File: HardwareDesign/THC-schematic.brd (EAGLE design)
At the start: 45 x 83 mm, 41 parts

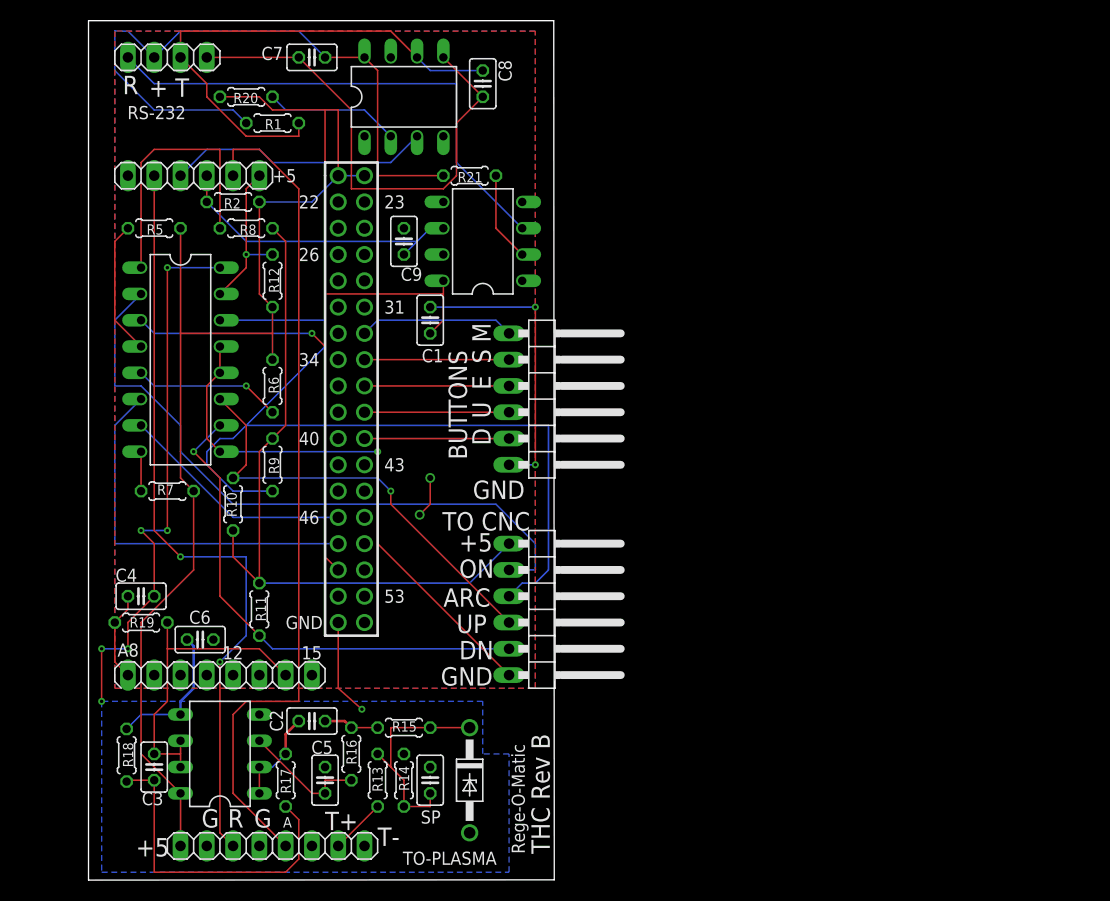
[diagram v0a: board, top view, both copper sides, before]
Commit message: Rev C Hardware
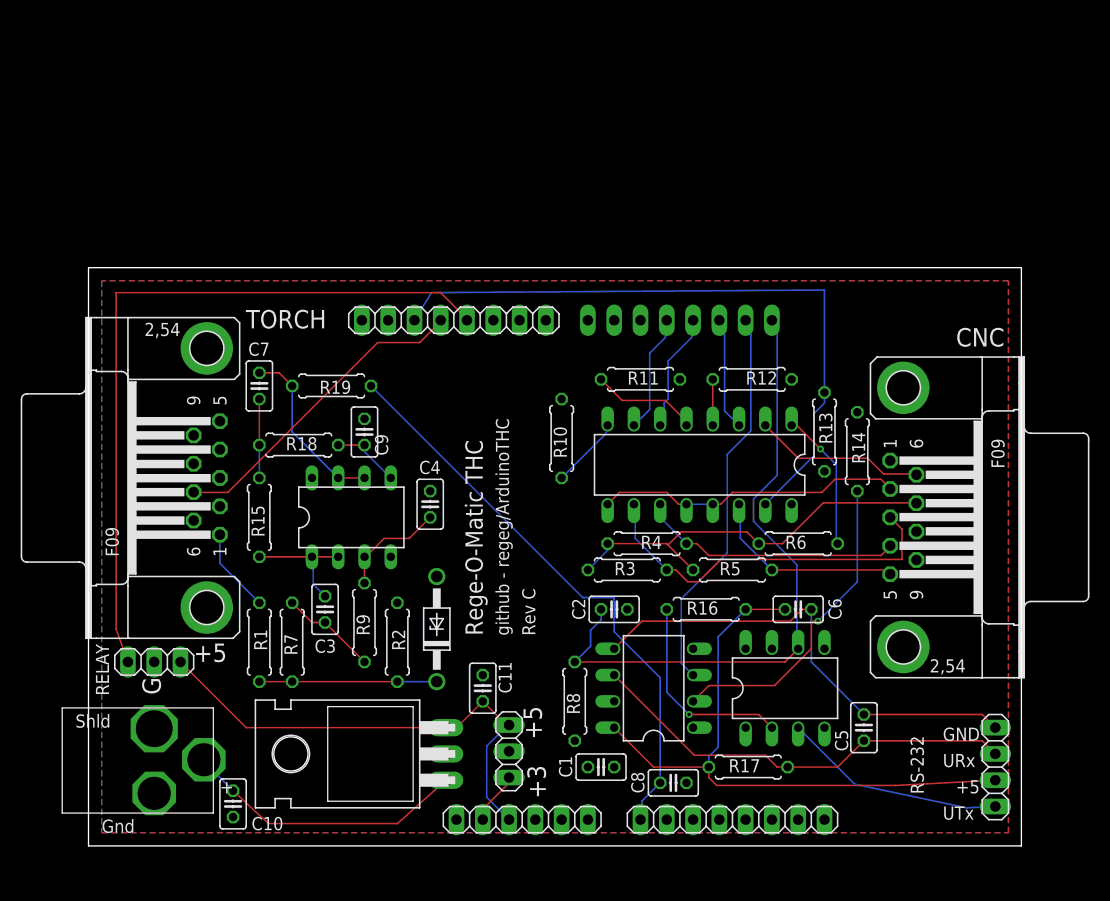
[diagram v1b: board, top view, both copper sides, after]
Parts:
- removed ARDUNIO-COMM: JJ, pinhead:1X06
- removed BUTTONS: CON1, pinhead:1X06/90
- removed MEGA-IO: ARDUINO-MEGA-18X2, ArduinoConnect18x2:CONN-18X2
- removed OK4: 6N137, optocoupler:DIL08
- removed R20, R21: 560, resistor:0204/5
- removed SP: 0, resistor:C025-025X050
- removed TO-CNC: CON3, pinhead:1X06/90
- removed TO-PLASMA: J1, pinhead:1X08
- removed U$2: LT1632, ArduinoThcOpAmp:DIP08
- added ARD-ANALOG, ARD-PWM, JP1: (no value), pinhead:1X08
- added ARD-PWR: (no value), pinhead:1X06
- added C10: 100nF / .1 uF, resistor:C025-025X050
- added C11: 100 nF / .1 uF, resistor:C025-025X050
- added CNC, TORCH: (no value), con-subd:F09HP
- added IC1: 7805T, adafruit:TO220H
- added ILQ2: ILQ1, optocoupler:DIL16
- added J1: 2.1MM-PLUG-PCB-MNT, ArdunioPowerJack:2.1MM-PLUG
- added JP2, RELAY: (no value), pinhead:1X03
- added R3, R4: 1k, resistor:0207/7
- C1: value .1uF -> 100 nF / 0.1uF
- C2: value 150n -> 15pf
- C3: value 1u -> 150 nf
- C4: value 10uF -> 100 nf / 0.1 uF
- C5: value 100n -> 15pf
- C6: value 100n -> 100 nF / 0.1uF
- C7: value .1uF -> 1 uF
- C8: value 15pf -> 10 uF
- C9: value 15pf -> 100 nf
- OK2: value ILQ1 -> 6N137; device optocoupler:DIL16 -> optocoupler:DIL08
- R1: value 350 -> 220k; device resistor:0204/5 -> resistor:0207/7
- R10, R11, R12: value 1k -> 560; device resistor:0204/5 -> resistor:0207/7
- R13: value 220k -> 1k; device resistor:0204/5 -> resistor:0207/7
- R14: value 15k -> 560; device resistor:0204/5 -> resistor:0207/7
- R15: value 7.87k -> 2.61k; device resistor:0204/5 -> resistor:0207/7
- R16: value 21.5k -> 560; device resistor:0204/5 -> resistor:0207/7
- R17: value 2.61k -> 350; device resistor:0204/5 -> resistor:0207/7
- R18, R19, R6: device resistor:0204/5 -> resistor:0207/7
- R2: value 350 -> 15k; device resistor:0204/5 -> resistor:0207/7
- R5: value 560 -> 1k; device resistor:0204/5 -> resistor:0207/7
- R7: value 560 -> 7.87k; device resistor:0204/5 -> resistor:0207/7
- R8: value 560 -> 350; device resistor:0204/5 -> resistor:0207/7
- R9: value 1k -> 21.5k; device resistor:0204/5 -> resistor:0207/7
- U$1: value PIN-ARD-A8 -> LT1632; device Rege:A8-1X8 -> ArduinoThcOpAmp:DIP08
- moved RS-232 105.4 mm to (87.6, 7.62), turned to 90 degrees
- moved C8 70.0 mm to (56.5, 6.10), turned to 0 degrees
- moved OK2 66.5 mm to (67.3, 15.2), turned to 0 degrees
- moved R5 64.9 mm to (62.2, 26.7)
- moved OK3 62.0 mm to (54.6, 15.2), turned to 90 degrees
- moved C6 57.9 mm to (68.6, 22.9)
- moved R8 55.7 mm to (47.0, 14.0), turned to 90 degrees
- moved R13 54.7 mm to (71.1, 40.0), turned to 270 degrees
- moved R14 54.1 mm to (74.3, 38.1)
- moved R6 53.0 mm to (68.6, 29.2), turned to 0 degrees
- moved C5 52.3 mm to (74.9, 11.4)
- moved R1 50.2 mm to (16.5, 19.7), turned to 270 degrees
- moved R12 47.3 mm to (64.1, 45.1), turned to 0 degrees
- moved C1 46.2 mm to (49.5, 7.62), turned to 0 degrees
- moved R2 45.4 mm to (29.8, 19.7), turned to 270 degrees
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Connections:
- removed net N$14: BUTTONS.1, MEGA-IO.D-33
- removed net N$15: BUTTONS.2, MEGA-IO.D-35
- removed net N$17: MEGA-IO.D-50, OK2.3
- removed net N$18: MEGA-IO.D-48, OK2.6
- removed net N$19: MEGA-IO.D-46, OK2.7
- removed net N$23: BUTTONS.3, MEGA-IO.D-37
- removed net N$24: BUTTONS.4, MEGA-IO.D-39
- removed net N$25: BUTTONS.5, MEGA-IO.D-41
- removed net N$28: C4.1, R19.1, U$1.1
- new net +3.3V: ARD-PWR.5, JP2.3
- new net ARC-GOOD-ARD: ILQ2.3, JP1.3
- new net ARD-ANALOG-IN: ARD-ANALOG.1, C8.1, R19.1
- new net N$1: C10.1, IC1.1, J1.P$POS
- new net TORCH-DOWN-ARD: ILQ2.7, JP1.5
- new net TORCH-UP-ARD: ILQ2.6, JP1.4
- new net VCC: C1.1, JP2.2, OK2.8, R10.2, R11.2, R12.2, R13.2, R14.1, R8.1, U$1.8
- net +5V: now also ARD-PWR.4, C11.1, IC1.3, JP2.1, RELAY.1; no longer C1.1, MEGA-IO.+5, MEGA-IO.+5V, OK4.8, R12.2, R2.1, R20.1, R5.2, R6.2, R7.2, TO-PLASMA.8, U$2.8
- net ARC-OK-INT: now also ARD-PWM.4, TORCH.7; no longer ARDUNIO-COMM.2, TO-PLASMA.4
- net ARDUINO-RX: now also C2.1, JP1.1, OK2.6, R8.2; no longer ARDUNIO-COMM.3, C9.1, OK4.6, R2.2
- net ARDUINO-TX: now also JP1.2; no longer ARDUNIO-COMM.4
- net CNC-GND: now also CNC.2, ILQ2.12, ILQ2.13, ILQ2.9; no longer OK2.12, OK2.13, OK2.9, TO-CNC.6
- net DIVIDER: now also R1.2, R2.2, R7.1; no longer R13.2, R14.2, R15.1, SP.1
- net GND: now also ARD-PWM.2, ARD-PWR.2, ARD-PWR.3, C10.2, C11.2, C2.2, C8.2, CNC.G1, IC1.2, ILQ2.16, J1.P$NEG, J1.P$SHLD, OK2.5, R2.1, RELAY.2, TORCH.5, TORCH.6, TORCH.G1, U$1.4; no longer BUTTONS.6, C5.2, C6.2, MEGA-IO.GND, MEGA-IO.GND-, OK2.16, OK4.5, R14.1, SP.2, TO-PLASMA.1, TO-PLASMA.5, TO-PLASMA.7, U$2.4
- net N$10: now also CNC.5, ILQ2.14, R5.2; no longer OK2.14, R9.2, TO-CNC.3
- net N$11: now also CNC.4, ILQ2.11, R4.2; no longer OK2.11, R10.2, TO-CNC.4
- net N$12: now also CNC.3, ILQ2.10, R3.2; no longer OK2.10, R11.2, TO-CNC.5
- net N$16: now also CNC.6, ILQ2.2; no longer OK2.2, TO-CNC.2
- net N$2: now also ILQ2.4, R12.1; no longer OK2.4, R5.1
- net N$22: now also CNC.7, R3.1, R4.1, R5.1, R6.1; no longer R10.1, R11.1, R8.1, R9.1, TO-CNC.1
- net N$26: now also C3.2, R7.2, R9.1; no longer C2.2, R15.2, R16.1
- net N$27: now also C4.1, R9.2, U$1.3; no longer C5.1, R16.2, U$2.3
- net N$29: now also C3.1, R15.1, U$1.1, U$1.2; no longer C2.1, R17.1, U$2.1, U$2.2
- net N$30: now also C7.1, R15.2; no longer C3.1, R17.2
- net N$31: now also C9.1, U$1.5; no longer C6.1, U$2.5
- net N$32: now also R14.2; no longer R20.2
- net N$34: now also OK2.2, R16.1; no longer OK4.2, R21.1
- net N$7: now also ILQ2.5, R11.1; no longer OK2.5, R6.1
- net N$8: now also ILQ2.8, R10.1; no longer OK2.8, R7.1
- net N$9: now also ILQ2.1, R6.2; no longer OK2.1, R8.2
- net SERIAL+5V: now also C6.1, R16.2, R17.1; no longer C7.1, R1.1, R21.2
- net SERIAL-GND: now also C5.2, C6.2; no longer C7.2, C8.2
- net TORCH+: now also R1.1, TORCH.1; no longer R13.1, TO-PLASMA.2
- net TORCH-ON-INT: now also ARD-PWM.3, ILQ2.15, R13.1; no longer ARDUNIO-COMM.1, OK2.15, R12.1
- net TORCH-ON-RELAY: now also ARD-PWM.5, RELAY.3; no longer ARDUNIO-COMM.5, TO-PLASMA.6
- net UNFILTERED: now also C7.2, U$1.6; no longer C3.2, U$2.6, U$2.7
- net USB-RX: now also C5.1, R17.2; no longer C8.1, R1.2
- net USB-TX: now also OK2.3; no longer OK4.3
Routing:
- net +5V: track 152.9 -> 47.4 mm
- net GND: track 91.0 -> 0.00 mm, vias 9 -> 0
- net N$10: track 85.1 -> 19.3 mm
- net ARD-ANALOG-IN: track 0.00 -> 56.1 mm
- net ARC-OK-INT: track 81.7 -> 30.9 mm
- net TORCH-ON-INT: track 15.5 -> 64.2 mm, vias 1 -> 0
- net N$16: track 63.5 -> 16.6 mm
- net N$17: track 40.9 -> 0.00 mm, vias 1 -> 0
- net N$18: track 36.6 -> 0.00 mm
- net ARDUINO-RX: track 29.3 -> 62.9 mm
- net N$22: track 67.7 -> 39.3 mm
- net USB-TX: track 49.4 -> 21.6 mm
- net N$30: track 31.7 -> 7.62 mm
- net CNC-GND: track 53.3 -> 29.7 mm, vias 1 -> 0
- net N$1: track 4.34 -> 27.6 mm, vias 2 -> 0
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- added copper zone on layer 1, net VCC
- removed copper zone on layer 1, net +5
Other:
- board size 45 x 83 mm -> 90.2 x 55.9 mm
- board text added: "+3"
- board text added: "Rege-O-Matic THC"
- board text added: "Rev C"
- board text added: "URx"
- board text added: "UTx"
- board text added: "github - regeg/ArduinoTHC"
- board text removed: "+"
- board text removed: "A"
- board text removed: "ARC"
- board text removed: "BUTTONS"
- board text removed: "D"
- board text removed: "DN"
- board text removed: "E"
- board text removed: "M"
- board text removed: "ON"
- board text removed: "R"
- board text removed: "Rege-O-Matic"
- board text removed: "S"
- board text removed: "T"
- board text removed: "T+"
- board text removed: "T-"
- board text removed: "THC Rev B"
- board text removed: "TO CNC"
- board text removed: "U"
- board text removed: "UP"
